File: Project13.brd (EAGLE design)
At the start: 27.6 x 50.8 mm, 3 parts, among them J1 CONNECTOR-19--1-TO-19, J2 CONNECTOR-19--20-TO-38, U1 BM20SPKA1NBC-0001AA

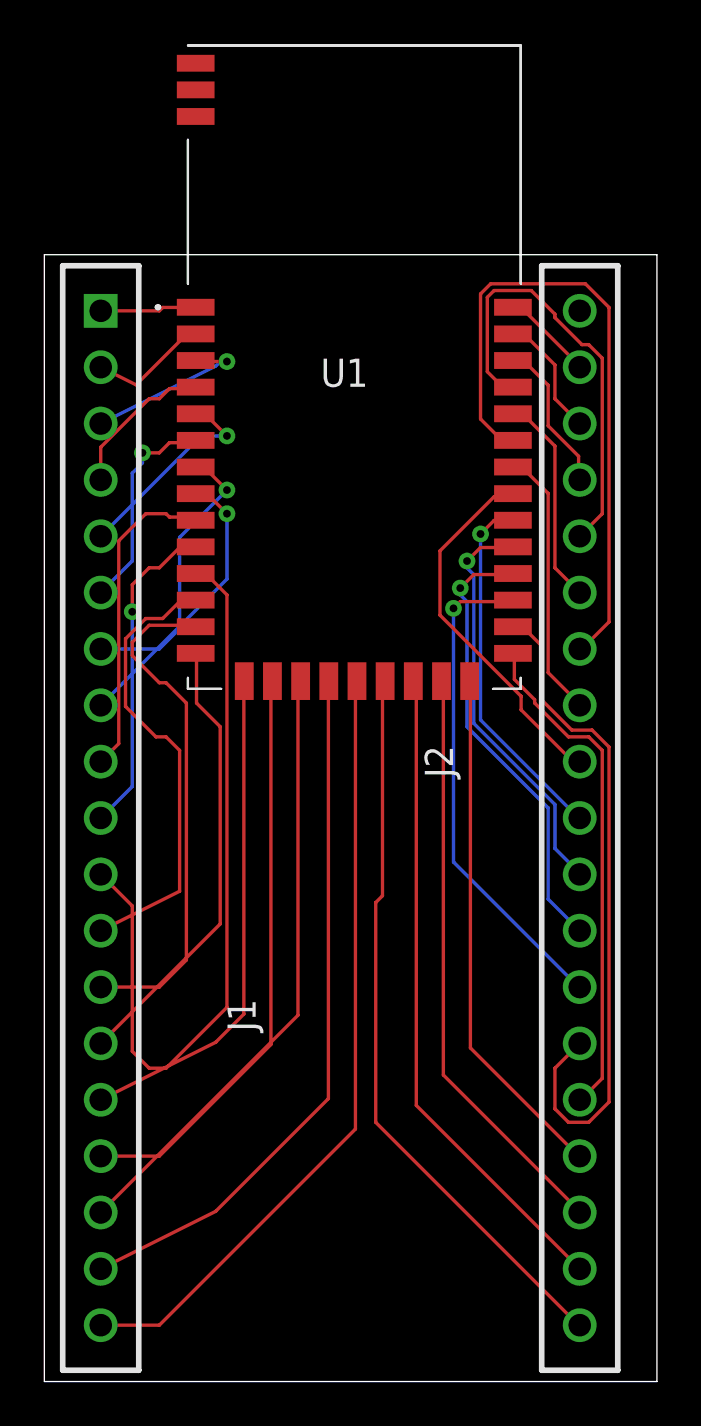
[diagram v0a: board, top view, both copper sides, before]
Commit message: Add files via upload
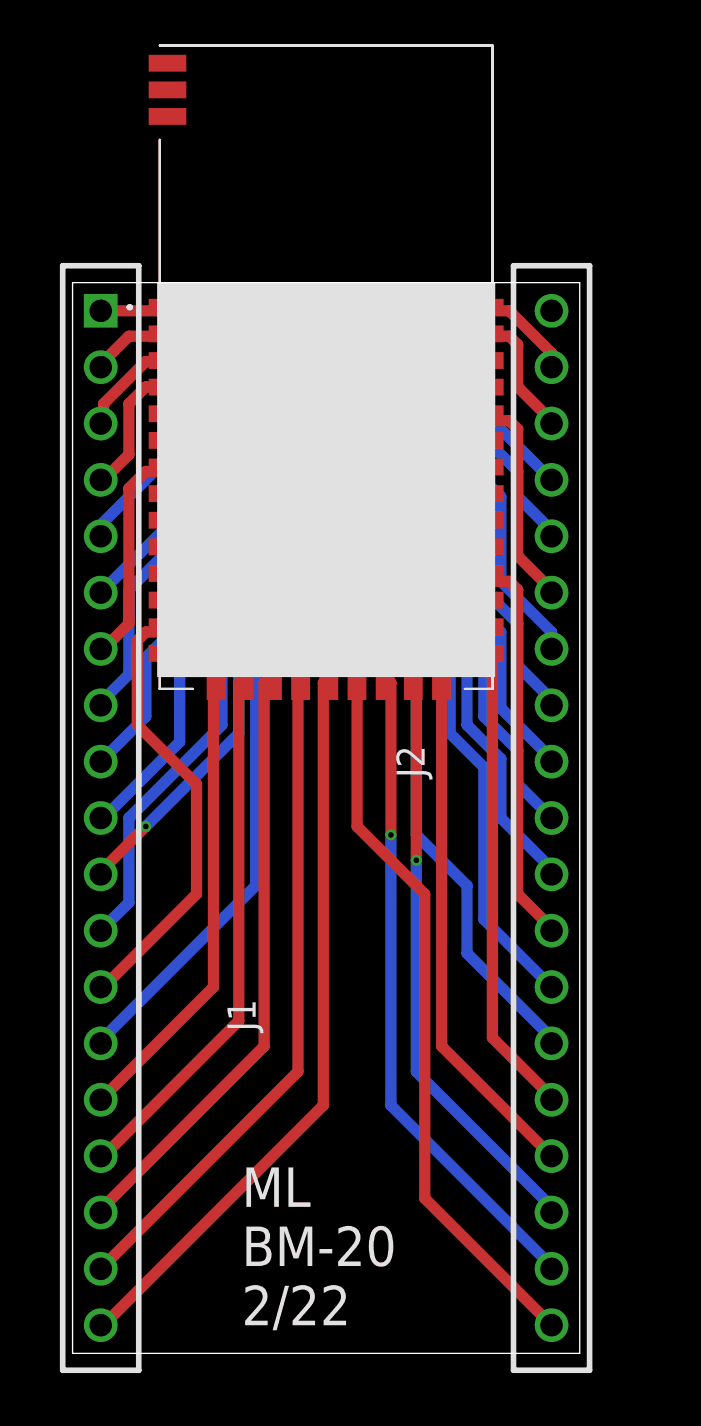
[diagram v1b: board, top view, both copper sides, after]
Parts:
- moved U1 1.27 mm to (12.7, 47.0)
- moved J2 1.27 mm to (22.9, 26.7)
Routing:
- net N$31: track 29.9 -> 12.8 mm, vias 0 -> 1
- net N$11: track 34.7 -> 18.1 mm, vias 0 -> 2
- net N$33: track 19.9 -> 9.74 mm, vias 0 -> 1
- net N$23: track 30.5 -> 23.9 mm, vias 0 -> 1
- net N$14: track 20.3 -> 24.7 mm, vias 0 -> 1
- net N$6: track 7.82 -> 4.62 mm, vias 1 -> 0
- net N$7: track 12.9 -> 9.97 mm, vias 1 -> 0
- net N$13: track 23.1 -> 20.2 mm
- net N$26: track 20.3 -> 17.8 mm, vias 1 -> 0
- net N$30: track 12.2 -> 14.2 mm, vias 0 -> 1
- net N$16: track 26.2 -> 24.2 mm
- net N$19: track 35.4 -> 33.4 mm
- net N$4: track 5.41 -> 3.66 mm
- net N$12: track 20.5 -> 18.8 mm, vias 0 -> 1
- net N$18: track 31.8 -> 30.2 mm
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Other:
- board size 27.6 x 50.8 mm -> 22.9 x 48.3 mm
- board text added: "ML BM-20 2/22"
